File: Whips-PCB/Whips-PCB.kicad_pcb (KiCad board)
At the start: 2 copper layers, 82 x 86 mm, 33 parts, among them J1 12 VDC, J2 RS422 BUS, J3 SPEAKER 4OHM, J4 TO WHIP, J5 RS422 BUS, SW2 SW_DIP_x06, U2 MAX485ESA+T, U3 SN74AHCT125DR, U4 TSR_1-2450, U5 MAX98357AETE+T, U6 Teensy4.1_Minimal

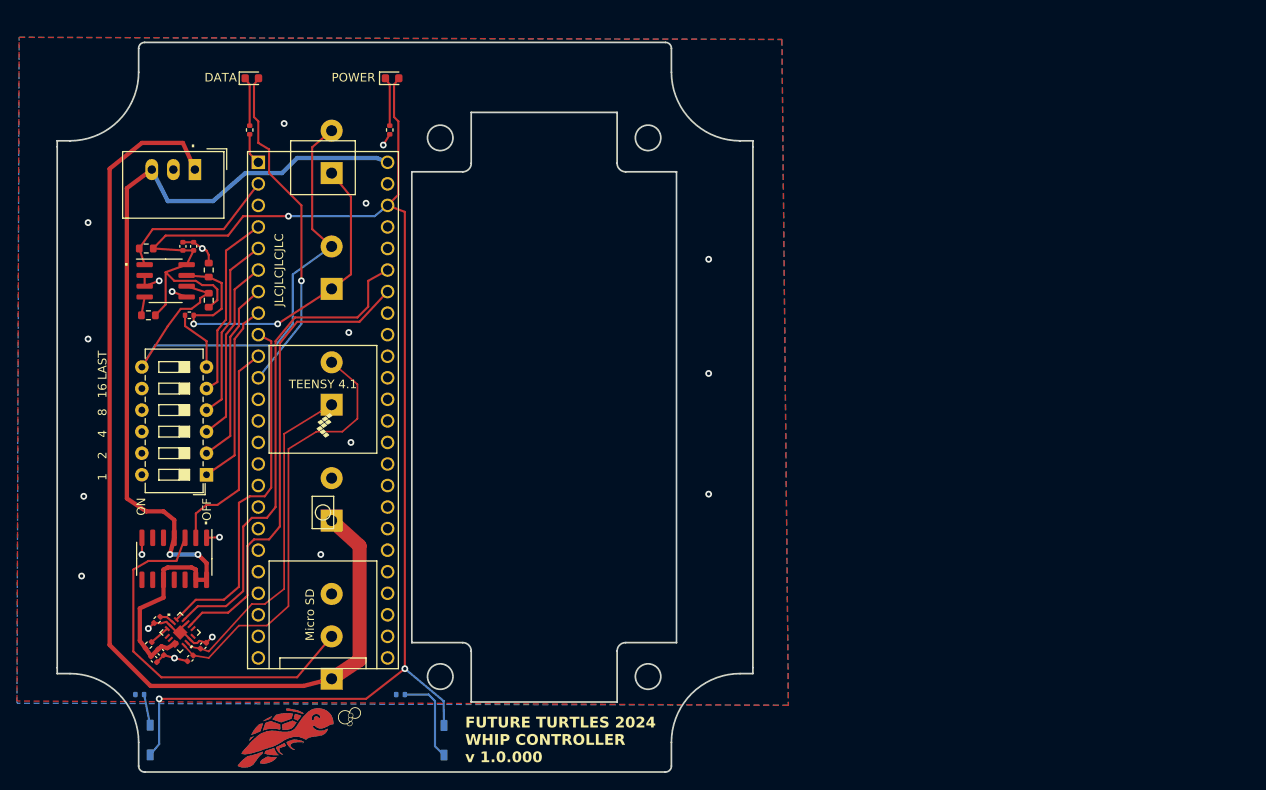
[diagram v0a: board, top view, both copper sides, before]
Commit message: Antenna 2026 initiated; new controller PCB
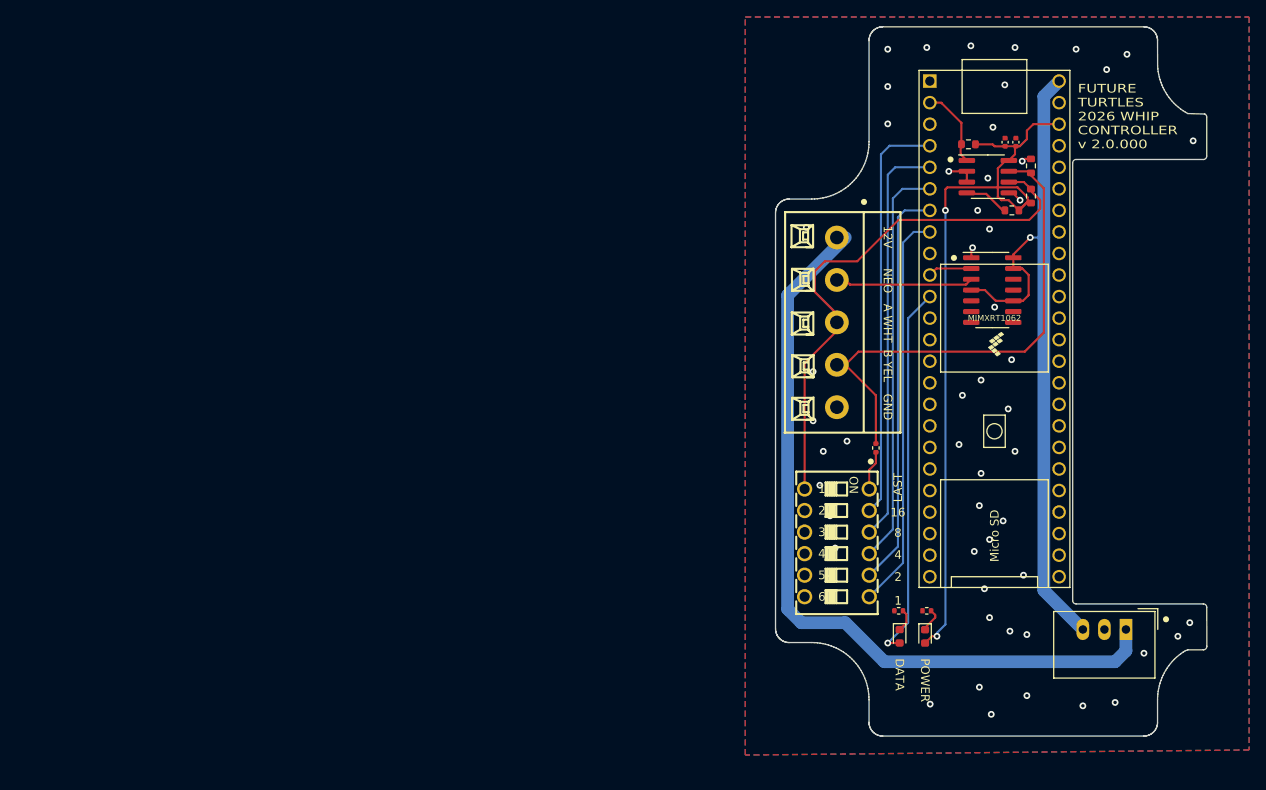
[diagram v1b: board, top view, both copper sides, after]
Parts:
- removed C4: 0.1uF, Capacitor_SMD:C_0402_1005Metric
- removed C5: 10uF, Capacitor_SMD:C_0402_1005Metric
- removed C6, C7: 220pF, Capacitor_SMD:C_0402_1005Metric
- removed D3, D4: LED, Joels KiCad Footprint Library:Everlight 99-218GLM2C-L7277SGU-TR8-T0-ES side view LED
- removed H1: DNP (LOGO), Joels KiCad Footprint Library:Turtle-Art-2024
- removed J1: 12 VDC, TerminalBlock_Phoenix:TerminalBlock_Phoenix_MKDS-1,5-2_1x02_P5.00mm_Horizontal
- removed J3: SPEAKER 4OHM, TerminalBlock_Phoenix:TerminalBlock_Phoenix_MKDS-1,5-2_1x02_P5.00mm_Horizontal
- removed J4: TO WHIP, TerminalBlock_Phoenix:TerminalBlock_Phoenix_MKDS-1,5-3_1x03_P5.00mm_Horizontal
- removed J5: RS422 BUS, TerminalBlock_Phoenix:TerminalBlock_Phoenix_MKDS-1,5-2_1x02_P5.00mm_Horizontal
- removed R10, R11: 470, Resistor_SMD:R_0402_1005Metric
- removed R7: 1M, Resistor_SMD:R_0402_1005Metric
- removed R8: 100K, Resistor_SMD:R_0402_1005Metric
- removed SW2: SW_DIP_x06, Button_Switch_THT:SW_DIP_SPSTx06_Slide_6.7x16.8mm_W7.62mm_P2.54mm_LowProfile
- removed U5: MAX98357AETE+T, Joels KiCad Footprint Library:MAX98357AETE+T
- added SW1: DSWB06LHGET, Joels KiCad Footprint Library:DongGuan_DSWB06LHGET_6_PIN_DIP, F.Cu at (176.4, 110.4)
- J2: value RS422 BUS -> Conn_01x05_Socket; footprint TerminalBlock_Phoenix:TerminalBlock_Phoenix_MKDS-1,5-2_1x02_P5.00mm_Horizontal -> Joels KiCad Footprint Library:Dorabo_DB103-5.0-5P-GN-S; moved to F.Cu
- moved U4 122.4 mm to (210.5, 120.6)
- moved R3 102.5 mm to (197.0, 71.2)
- moved U3 101.5 mm to (194.7, 80.6), turned to 0 degrees
- moved D2 100.8 mm to (183.8, 121.4), turned to -90 degrees
- moved C1 97.7 mm to (197.5, 63.2)
- moved C2 97.7 mm to (196.2, 63.2)
- moved R1 97.7 mm to (199.3, 69.5)
- moved R2 97.7 mm to (199.3, 66.0)
- moved R4 97.7 mm to (191.9, 63.4)
- moved U2 97.7 mm to (194.2, 67.2)
- moved R9 95.2 mm to (183.7, 118.4), turned to 180 degrees
- moved D1 91.0 mm to (186.8, 121.4), turned to -90 degrees
- moved R6 85.0 mm to (187.0, 118.4), turned to 180 degrees
- moved R5 82.4 mm to (181.0, 99.2), turned to 90 degrees
- moved U6 79.7 mm to (195.0, 85.2)
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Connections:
- J2 pad 1: /B -> /12VDC
- J2 pad 2: /A -> /NEO
- R1 pad 2: /A -> /RS422-A
- R2 pad 2: /B -> /RS422-B
- R5 pad 2: /B -> /RS422-B
- U2 pad 6: /A -> /RS422-A
- U2 pad 7: /B -> /RS422-B
- U6 pad 42: /LRCLK -> unconnected-(U6-20_A6_TX5_LRCLK1-Pad42)
- U6 pad 43: /BCLK -> unconnected-(U6-21_A7_RX5_BCLK1-Pad43)
- U6 pad 9: /DAT -> unconnected-(U6-7_RX2_OUT1A-Pad9)
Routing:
- net +3.3V: track 172.1 -> 91.1 mm, vias 3 -> 2
- net /RS422-A: track 0.00 -> 64.5 mm
- net /A: track 62.9 -> 0.00 mm
- net /BCLK: track 58.7 -> 0.00 mm
- net /RS422-B: track 0.00 -> 57.9 mm
- net /LRCLK: track 55.9 -> 0.00 mm
- net /VO+: track 51.3 -> 0.00 mm
- net /B: track 45.0 -> 0.00 mm, vias 2 -> 0
- net /DAT: track 42.3 -> 0.00 mm
- net /VO-: track 39.7 -> 0.00 mm
- net /NEO: track 44.7 -> 15.3 mm
- net /12VDC: track 119.4 -> 92.1 mm
- net +5V: track 112.2 -> 85.4 mm, vias 2 -> 1
- net Net-(U6-2_OUT2): track 22.1 -> 48.7 mm
- net Net-(U6-3_LRCLK2): track 22.0 -> 48.3 mm
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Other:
- board size 82 x 86 mm -> 50.8 x 83.6 mm
- board text added: "A WHT"
- board text added: "B YEL"
- board text added: "FUTURE TURTLES 2026 WHIP CONTROLLER v 2.0.000"
- board text added: "NEO"
- board text removed: "."
- board text removed: "DAT"
- board text removed: "DSH"
- board text removed: "FUTURE TURTLES 2024 WHIP CONTROLLER v 1.0.000"
- board text removed: "OFF"
- board text removed: "ON"
- board text removed: "RS422"
- board text removed: "SLD"
- board text removed: "SPEAKER"
- board text removed: "TO WHIP"
